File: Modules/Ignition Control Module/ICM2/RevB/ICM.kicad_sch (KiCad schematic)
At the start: 7 parts, among them J1 Conn_01x06, Q1 ISL9V3040P3, Q2 ISL9V3040P3

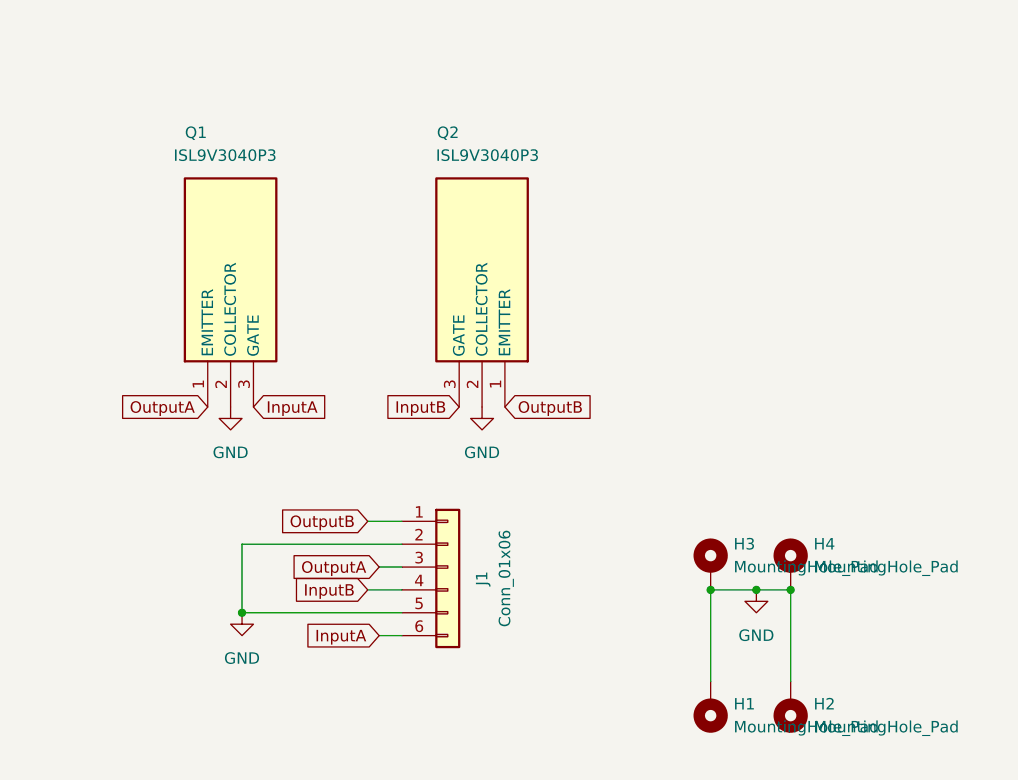
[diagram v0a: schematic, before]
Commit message: Reorganization - Version uploads
CDx4 B1,2 - NCV1124 B3 - PMAPM 2 - Sim8 B3 - Upload
Remove ICM2A (design issues), Upload ICM2B Major redesign,
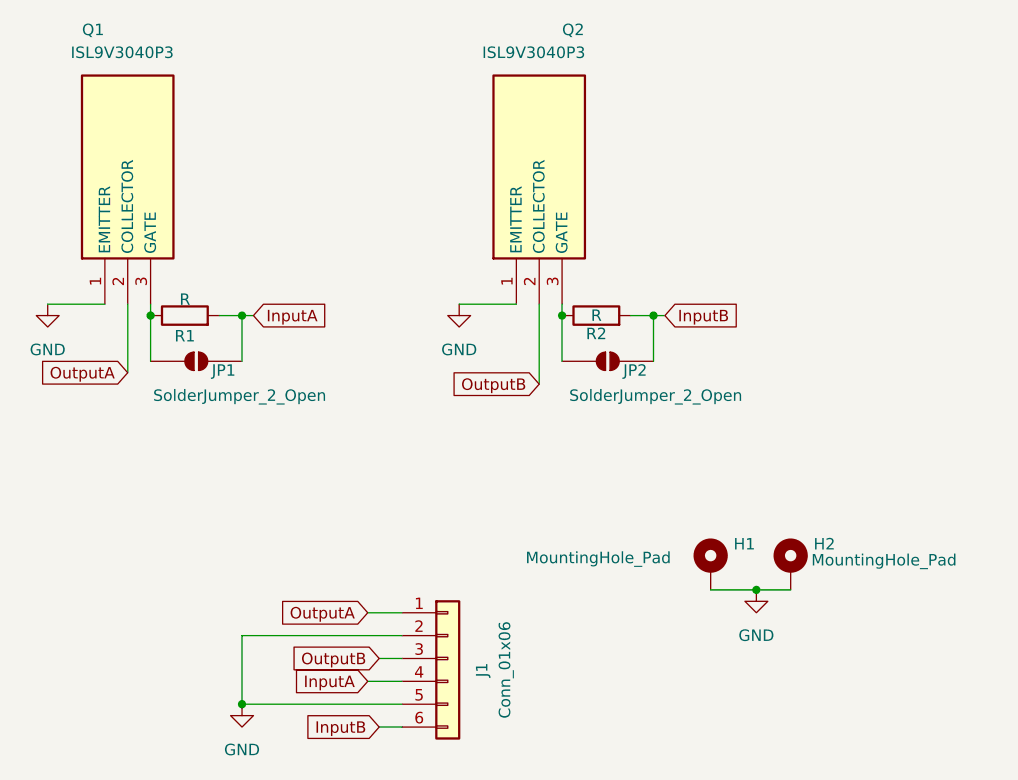
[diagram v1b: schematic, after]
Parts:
- removed H1, H4: MountingHole_Pad, MountingHole:MountingHole_4.3mm_M4_DIN965_Pad, symbol Mechanical:MountingHole_Pad
- added JP1, JP2: SolderJumper_2_Open, Jumper:SolderJumper-2_P1.3mm_Bridged_RoundedPad1.0x1.5mm, symbol Jumper:SolderJumper_2_Open
- added R1, R2: R, Resistor_THT:R_Axial_DIN0207_L6.3mm_D2.5mm_P10.16mm_Horizontal, symbol Device:R
- H1: renamed from H3; footprint MountingHole:MountingHole_4.3mm_M4_DIN965_Pad -> MountingHole:MountingHole_3.2mm_M3_DIN965_Pad_TopBottom
- H2: footprint MountingHole:MountingHole_4.3mm_M4_DIN965_Pad -> MountingHole:MountingHole_3.2mm_M3_DIN965_Pad_TopBottom
- J1: footprint Connector_Molex:Molex_Micro-Fit_3.0_43045-0600_2x03_P3.00mm_Horizontal -> Connector_Molex:Molex_Mini-Fit_Jr_5569-06A2_2x03_P4.20mm_Horizontal
- Q1, Q2: footprint Package_TO_SOT_THT:TO-220-3_Horizontal_TabDown -> Detonation:TO-252-2-frontThermalOnly; LCSC (none) -> C462128
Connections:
- net GND: now also Q1.1 (EMITTER), Q2.1 (EMITTER); no longer Q1.2 (COLLECTOR), Q2.2 (COLLECTOR)
- net InputA: now also J1.4 (Pin_4), JP1.2 (B), R1.2; no longer J1.6 (Pin_6), Q1.3 (GATE)
- net InputB: now also J1.6 (Pin_6), JP2.2 (B), R2.2; no longer J1.4 (Pin_4), Q2.3 (GATE)
- net OutputA: now also J1.1 (Pin_1), Q1.2 (COLLECTOR); no longer J1.3 (Pin_3), Q1.1 (EMITTER)
- net OutputB: now also J1.3 (Pin_3), Q2.2 (COLLECTOR); no longer J1.1 (Pin_1), Q2.1 (EMITTER)
- new net: JP1.1 (A), Q1.3 (GATE), R1.1
- new net: JP2.1 (A), Q2.3 (GATE), R2.1
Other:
- moved on the sheet: H2, Q1, Q2
